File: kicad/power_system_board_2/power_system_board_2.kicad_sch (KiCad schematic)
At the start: 21 parts, among them J1 USB_C_Receptacle_USB2.0_16P, J2 Conn_01x04_Pin, Q1 NMOS, Q3 PMOS, U1 ${SIM.PARAMS}

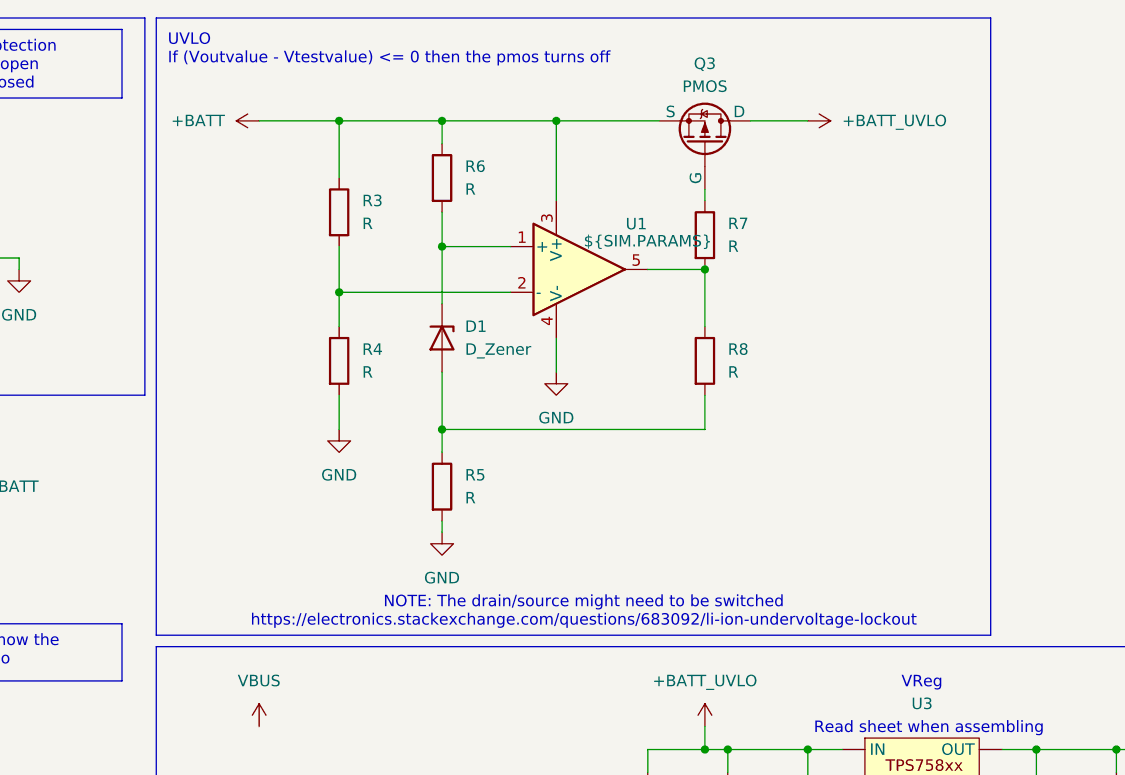
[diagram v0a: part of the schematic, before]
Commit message: Pushing a few more changes so I have everything
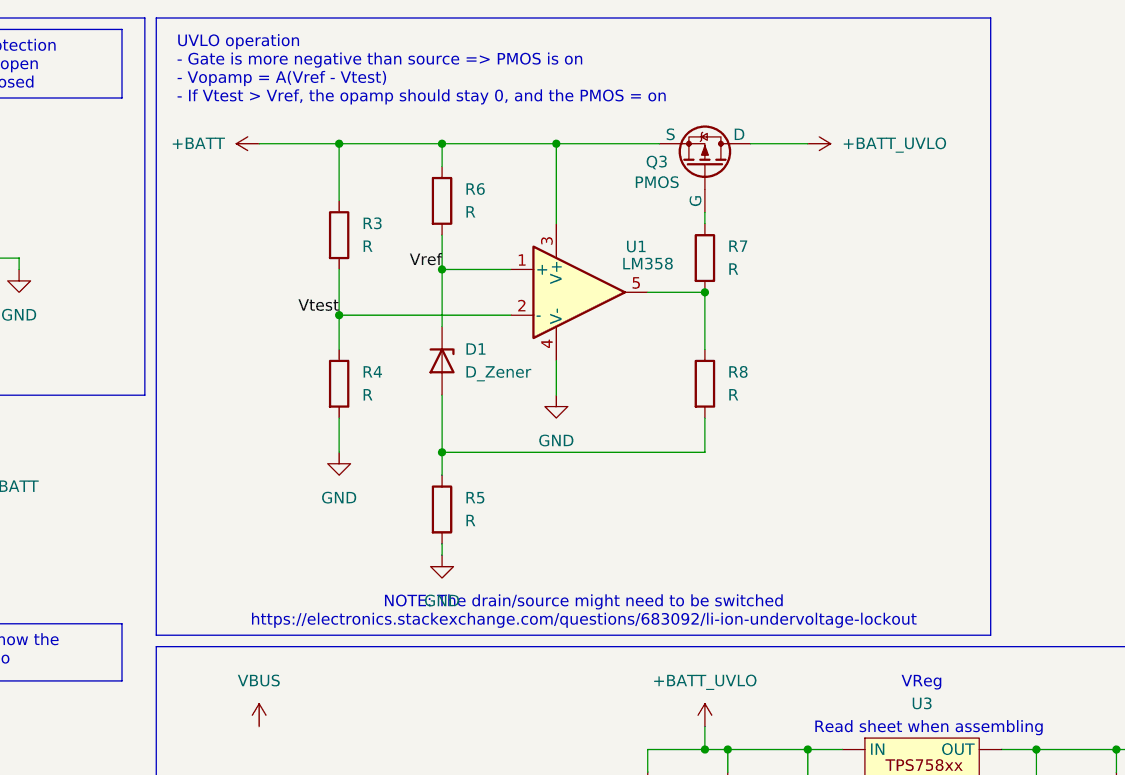
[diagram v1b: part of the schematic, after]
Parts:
- U1: value ${SIM.PARAMS} -> LM358
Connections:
- net Vtest: now reaches R3.2, R4.1, U1.2 (-)
- net Vref: now reaches D1.1 (K), R6.2, U1.1 (+)
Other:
- note added: "UVLO operation - Gate is more negative than source => PMOS is on - Vopamp = A(Vref - Vtest) - If Vtest > Vref, the opamp should stay 0, and the PMOS = on"
- note removed: "UVLO If (Voutvalue - Vtestvalue) <= 0 then the pmos turns off"
- moved on the sheet: D1, Q3, R3, R4, R5, R6, R7, R8, U1
